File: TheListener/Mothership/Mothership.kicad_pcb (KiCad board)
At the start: 2 copper layers, 65 parts, among them J1 RJ45, J2 RJ45, J3 RJ45, J4 RJ45, J5 RJ45, J6 RJ45, J7 RJ45, J8 RJ45, J9 Conn_01x02_Female, U1 SP3491, U10 AMS1117-3.3, U11 NID35-5, U12 Teensy3.5, U2 SP3491, U3 SP3491, U4 SP3491, U5 SP3491, U6 SP3491, U7 SP3491, U8 SP3491, U9 AMS1117-3.3

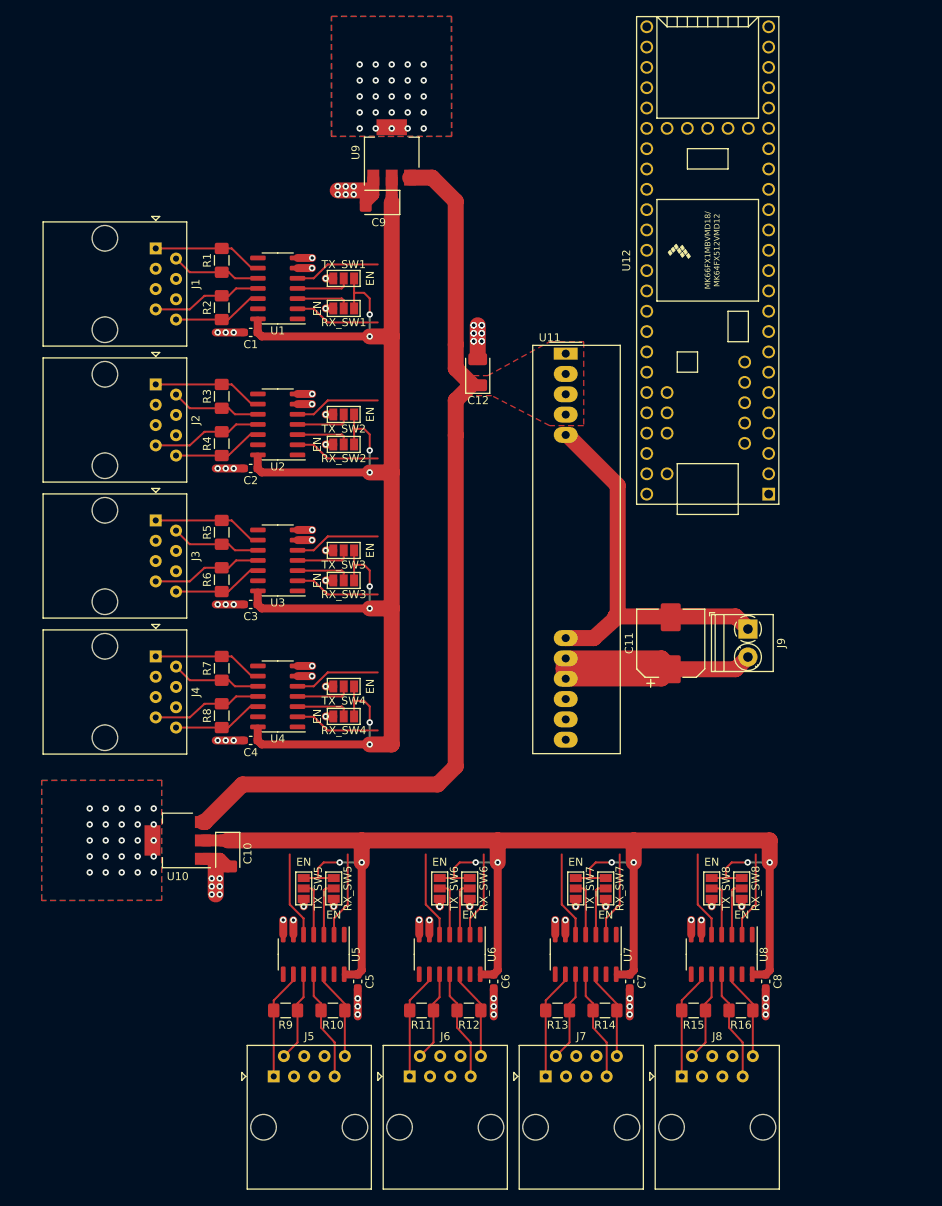
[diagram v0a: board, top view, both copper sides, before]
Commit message: all except signals; needs refinement of power
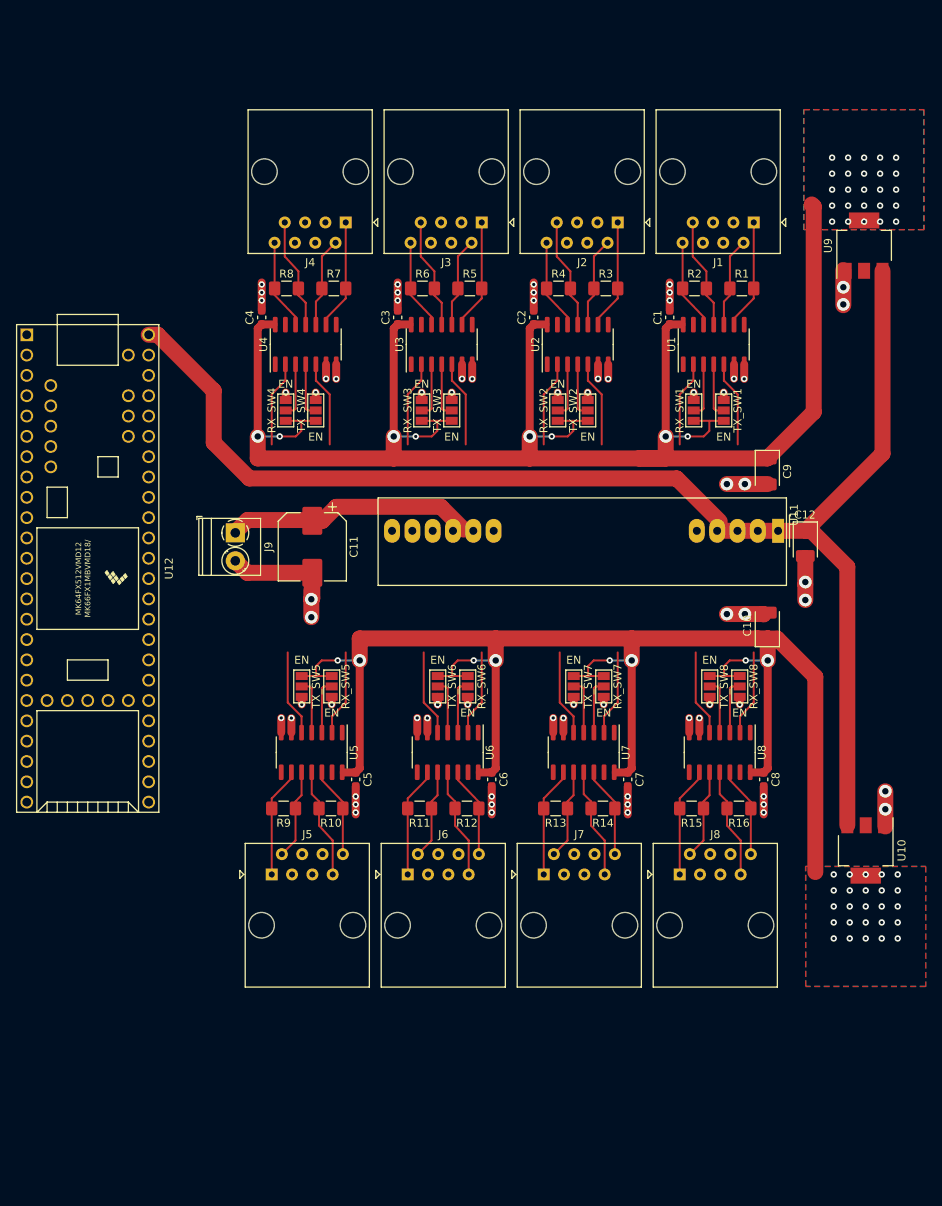
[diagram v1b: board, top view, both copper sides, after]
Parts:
- moved U12 86.5 mm to (26.2, 79.2), turned to 270 degrees
- moved U10 86.0 mm to (123.5, 114.5), turned to 270 degrees
- moved J1 74.8 mm to (109.5, 36.0), turned to 180 degrees
- moved C10 73.2 mm to (111.2, 86.4), turned to 90 degrees
- moved J9 65.2 mm to (44.7, 74.8)
- moved R1 65.1 mm to (108.0, 44.2), turned to 0 degrees
- moved J2 61.2 mm to (92.5, 36.0), turned to 180 degrees
- moved U9 60.2 mm to (123.3, 38.9)
- moved J4 59.2 mm to (58.5, 36.0), turned to 180 degrees
- moved R2 59.1 mm to (102.1, 44.2), turned to 0 degrees
- moved C9 59.1 mm to (111.2, 67.1), turned to 270 degrees
- moved J3 55.2 mm to (75.5, 36.0), turned to 180 degrees
- moved U1 54.9 mm to (104.5, 51.2), turned to 90 degrees
- moved R8 54.0 mm to (51.1, 44.2), turned to 0 degrees
- moved C4 52.9 mm to (48.0, 47.9), turned to 270 degrees
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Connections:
- J9 pad 1: GND -> +24V
- J9 pad 2: +24V -> GND
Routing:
- net +5V: track 113.7 -> 171.9 mm
- net VCC1: track 191.5 -> 221.9 mm
- net GND: track 142.7 -> 113.9 mm, vias 81 -> 69
- net +24V: track 53.6 -> 31.1 mm
- net VCC2: track 191.4 -> 204.0 mm
- removed copper zone on F.Cu, net +5V
